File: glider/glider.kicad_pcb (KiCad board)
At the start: 4 copper layers, 40 x 60 mm, 115 parts, among them J1 SENSOR_I2C, J10 DM3CS-SF, J11 SCH1, J12 IO, J13 SCH2, J14 SCH3, J15 SCH4, J16 SCH5, J17 SCH6, J18 SCH7, J2 USB_B_Micro, J20 CELL, J3 HPS_A, J4 DEBUG_NAV, J6 SCH8, J7 GPS_UART, J8 NCP_COM, J9 IMU_SPI, Q1 DMP1045UQ, Q2 2N7002E, Q3 2N7002E, Q4 DMT6008LFG, SW1 NAV_NRST, SW2 NAV_BOOT, U10 MIC5501-3.0YM5, U11 NTB0104, U12 RT6218A, U2 STM32G484RETx, U3 MIC5504-1.8YM5, U4 MCP73831-2-OT, U5 MS5637, U6 W25N01GVZEIG, U7 ICM-20948, U8 L96-M33, Y1 8MHz

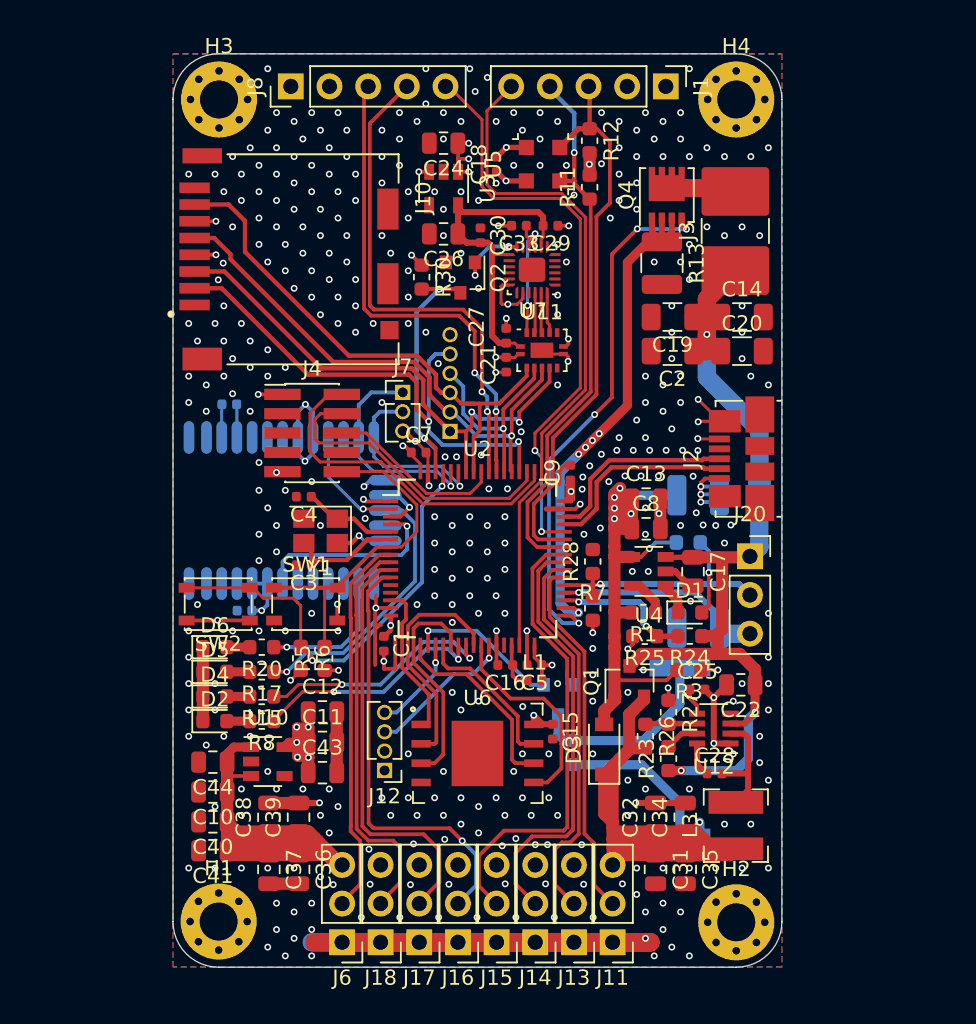
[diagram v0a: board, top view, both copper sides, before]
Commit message: submitted to jlc
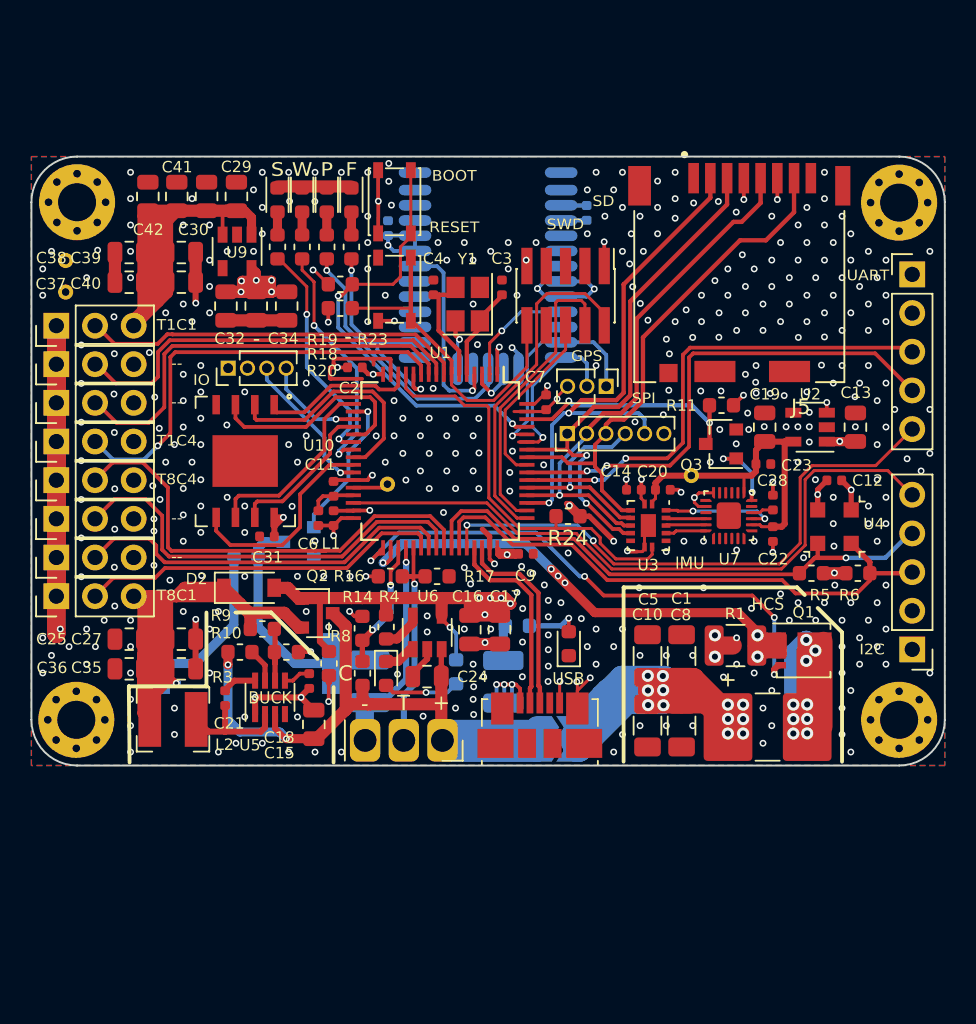
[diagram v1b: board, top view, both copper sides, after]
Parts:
- removed the C23 at (44.7, 146.6)
- removed the C25 at (74.5, 151.8)
- removed the C28 at (75.6, 157.3)
- removed the J3 at (76.9, 121.6)
- removed the R15 at (45.8, 152.2)
- removed the R18 at (43.7, 133.0)
- removed the R20 at (45.8, 149.0)
- removed R26: 100k, Resistor_SMD:R_0603_1608Metric
- removed the R8 at (45.8, 153.8)
- added C18: 0.1u, Capacitor_SMD:C_0402_1005Metric, F.Cu at (49.0, 151.2)
- added C21: 0.1u, Capacitor_SMD:C_0402_1005Metric, F.Cu at (43.4, 152.3)
- added C26: 0.1u, Capacitor_SMD:C_0402_1005Metric, B.Cu at (54.1, 121.5)
- added D7: SD1206T040S2R0, Diode_SMD:D_SOD-123, B.Cu at (79.1, 153.7)
- added D8: USB_PWR, LED_SMD:LED_0603_1608Metric, F.Cu at (66.0, 148.8)
- added J1: HPS_A, Resistor_SMD:R_2816_7142Metric_Pad3.20x4.45mm_HandSolder, F.Cu at (79.1, 154.2)
- added JP1: HPS_CELL_V, Jumper:SolderJumper-2_P1.3mm_Open_TrianglePad1.0x1.5mm, B.Cu at (65.1, 155.8)
- added N1: Bottom Graphic, atlas:boardartswift, B.Cu at (60.7, 136.7)
- added R12: 0, Resistor_SMD:R_0402_1005Metric, B.Cu at (67.2, 120.5)
- added R13: 100k, Resistor_SMD:R_0603_1608Metric, F.Cu at (52.5, 150.7)
- added R19: 1k, Resistor_SMD:R_0603_1608Metric, F.Cu at (46.9, 122.7)
- added R21: 1k, Resistor_SMD:R_0603_1608Metric, F.Cu at (48.5, 122.7)
- added R23: 1k, Resistor_SMD:R_0603_1608Metric, F.Cu at (51.7, 122.7)
- added R25: 1k, Resistor_SMD:R_0603_1608Metric, B.Cu at (62.6, 147.6)
- added R9: 100k, Resistor_SMD:R_0603_1608Metric, F.Cu at (45.9, 147.8)
- added TP1: VREFBUF, TestPoint:TestPoint_THTPad_D1.0mm_Drill0.5mm, B.Cu at (54.1, 138.3)
- added TP2: VCC_SYS, TestPoint:TestPoint_THTPad_D1.0mm_Drill0.5mm, B.Cu at (33.0, 125.7)
- added TP3: VDD_MCU, TestPoint:TestPoint_THTPad_D1.0mm_Drill0.5mm, B.Cu at (33.0, 123.6)
- added TP4: VDD_IMU, TestPoint:TestPoint_THTPad_D1.0mm_Drill0.5mm, B.Cu at (74.0, 137.7)
- D2: renamed from D3; value D_Schottky -> SD1206T040S2R0
- J18: renamed from J9; moved to F.Cu
- moved H1 48.2 mm to (33.7, 119.8), turned to 270 degrees
- moved H2 45.3 mm to (33.6, 153.8), turned to 270 degrees
- moved H3 45.2 mm to (87.7, 119.8), turned to 270 degrees
- moved J13 44.6 mm to (32.3, 127.9), turned to 90 degrees
- moved J12 43.5 mm to (32.3, 130.4), turned to 90 degrees
- moved C42 43.2 mm to (38.4, 119.4), turned to 90 degrees
- moved J6 43.0 mm to (32.3, 145.6), turned to 90 degrees
- moved J11 42.7 mm to (32.3, 132.9), turned to 90 degrees
- moved J17 42.6 mm to (88.6, 124.5), turned to 0 degrees
- moved J7 42.4 mm to (32.3, 143.1), turned to 90 degrees
- moved J10 42.2 mm to (32.3, 135.5), turned to 90 degrees
- moved H4 42.1 mm to (87.7, 153.8), turned to 270 degrees
- moved J8 42.0 mm to (32.3, 140.5), turned to 90 degrees
- moved J9 41.9 mm to (32.3, 138.0), turned to 90 degrees
- moved C38 41.6 mm to (37.1, 123.0), turned to 180 degrees
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- renumbered C19 to C1, C20 to C10, C16 to C11, C18 to C12, C24 to C13, C21 to C14, C22 to C15, C8 to C16, C13 to C17, C26 to C19, C1 to C2, C27 to C20, C29 to C22, C30 to C23, C17 to C24, C31 to C25, C32 to C27, C33 to C28, C44 to C29, C4 to C3, C10 to C30, C15 to C31, C11 to C32, C12 to C33, C43 to C34, C34 to C35, C35 to C36, C36 to C37, C37 to C38, C38 to C39, C3 to C4, C39 to C40, C40 to C41, C41 to C42, C2 to C5, C5 to C6, C14 to C8, D2 to D3, J16 to J10, J17 to J11, J18 to J12, J6 to J13, J1 to J14, J12 to J15, J7 to J16, J8 to J17, J4 to J2, J20 to J3, J2 to J4, J10 to J5, J11 to J6, J13 to J7, J14 to J8, J15 to J9, L3 to L2, Q4 to Q1, Q1 to Q2, Q2 to Q3, Q3 to Q4, R13 to R1, R27 to R10, R30 to R11, R25 to R14, R31 to R15, R7 to R16, R28 to R17, R6 to R18, R4 to R2, R5 to R20, R17 to R22, R23 to R3, R1 to R4, R11 to R5, R12 to R6, R2 to R7, R3 to R8, SW2 to SW1, SW1 to SW2, U2 to U1, U6 to U10, U3 to U2, U11 to U3, U5 to U4, U12 to U5, U4 to U6, U10 to U9
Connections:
- net /IMU_SPI2_MISO renamed /IMU_SPI3_MISO
- net /IMU_SPI2_MOSI renamed /IMU_SPI3_MOSI
- net /IMU_SPI2_SCK renamed /IMU_SPI3_SCK
- net Net-(C13-Pad1) renamed /VCC_USB
- R24 pad 1: /CELL_POS -> GND
- R24 pad 2: /OPAMP4_CELL_VS -> /IMU_SPI_LS_EN
- U1 pad 12: /HPS_B_TIM2_CH1 -> /GPS_FIX
- U1 pad 13: /HPS_B_OPAMP6_CS -> /IMU_SPI_LS_EN
- U3 pad 8: /VDD_MCU -> /IMU_SPI_LS_EN
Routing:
- net Net-(C1-Pad1): track 22.0 -> 74.6 mm, vias 1 -> 12
- net Net-(D7-Pad2): track 4.59 -> 41.9 mm, vias 0 -> 9
- net /IMU_SPI_LS_EN: track 0.00 -> 27.0 mm
- net /CELL_POS: track 39.7 -> 61.4 mm
- net /GPS_FIX: track 9.13 -> 15.5 mm, vias 1 -> 2
- net /VDD_SYS: track 148.1 -> 154.2 mm
- net /VDD_IMU: track 34.5 -> 29.4 mm
- net Net-(D8-Pad2): track 0.00 -> 3.68 mm, vias 0 -> 1
- net /VREFBUF_OUT: track 0.00 -> 2.37 mm
- net /HPS_A_OPAMP3_CS: track 36.7 -> 38.9 mm, vias 5 -> 6
- net GND: track 230.7 -> 228.5 mm, vias 407 -> 415
- net /VDD_MCU: track 60.6 -> 59.5 mm, vias 26 -> 23
- net /IMU_INT: track 16.8 -> 15.9 mm
- net /ADC2_IN15_CELL_TS: track 14.8 -> 15.7 mm
- net /VCC_USB: track 36.8 -> 36.0 mm
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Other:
- board size 40 x 60 mm -> 60 x 40 mm
- rule pad_to_mask_clearance: 0 -> 0.05
- rule via_min_size: 0.45 -> 0.4
- board text added: "+"
- board text added: "-"
- board text added: "--"
- board text added: "BOOT ~ RESET"
- board text added: "BUCK"
- board text added: "C"
- board text added: "F"
- board text added: "GPS"
- board text added: "HCS"
- board text added: "I2C"
- board text added: "IMU"
- board text added: "IO"
- board text added: "P"
- board text added: "S"
- board text added: "SD"
- board text added: "SPI"
- board text added: "SWD"
- board text added: "T"
- board text added: "T1C1"
- board text added: "T1C4"
- board text added: "T8C1"
- board text added: "T8C4"
- board text added: "UART"
- board text added: "USB"
- board text added: "W"
